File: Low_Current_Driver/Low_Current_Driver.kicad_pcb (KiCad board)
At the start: 4 copper layers, 160 x 99.5 mm, 194 parts, among them J1 Conn_01x02, J2 RJ45, J3 Screw_Terminal_01x04, J4 Conn_02x07_Odd_Even, J5 Channel 3, J6 Channel 2, J7 Channel 1, J8 MS548-10F, J9 Conn_01x02, Q1 Si4447ADY, Q2 IRF8707PbF, SW1 DPDT_Hirose, U1 LM4040DBZ-5, U10 OPA2210, U11 OPA2210, U12 OPA2210, U13 OPA2210, U14 OPA2210, U2 LM4040DBZ-5, U3 LM393, U4 TPS7A470x, U5 TPS7A470x, U6 TPS7A33, U7 LTC6655-2.5, U8 DAC8814, U9 OPA2210

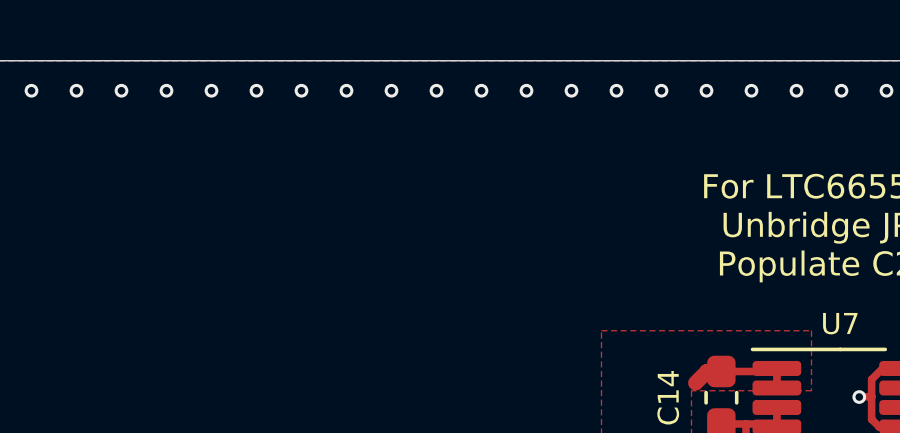
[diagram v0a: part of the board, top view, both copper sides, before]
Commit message: Revert "LCD amplifier update"
This reverts commit 83ce83a7733d65f451b9b157d86b817c7c87638f.
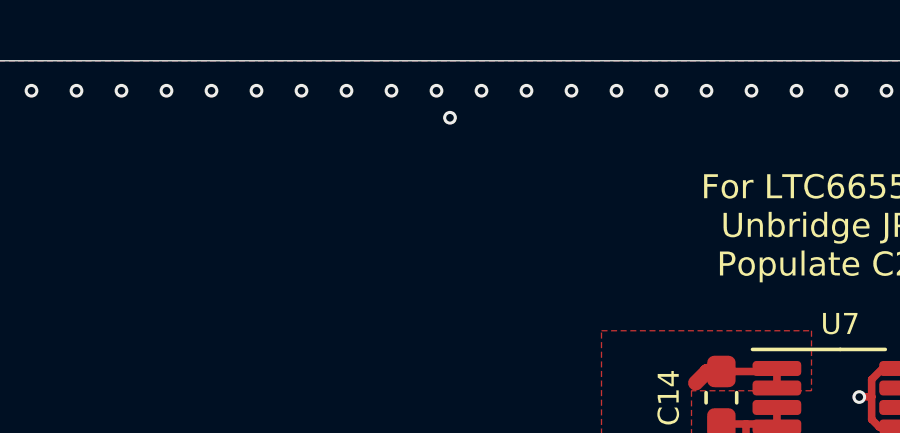
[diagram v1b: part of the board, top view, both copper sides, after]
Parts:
- U10, U11, U12, U13, U14, U9: value OPA2210 -> OPA2277
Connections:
- A1 pad 1: (no net) -> Net-(A1-Pad1)
- A1 pad 17: (no net) -> Net-(A1-Pad17)
- A1 pad 18: (no net) -> Net-(A1-Pad18)
- A1 pad 2: (no net) -> Net-(A1-Pad2)
- A1 pad 20: (no net) -> Net-(A1-Pad20)
- A1 pad 21: (no net) -> Net-(A1-Pad21)
- A1 pad 22: (no net) -> Net-(A1-Pad22)
- A1 pad 23: (no net) -> Net-(A1-Pad23)
- A1 pad 24: (no net) -> Net-(A1-Pad24)
- A1 pad 25: (no net) -> Net-(A1-Pad25)
- A1 pad 26: (no net) -> Net-(A1-Pad26)
- A1 pad 28: (no net) -> Net-(A1-Pad28)
- A1 pad 3: (no net) -> Net-(A1-Pad3)
- A1 pad 5: (no net) -> Net-(A1-Pad5)
- A1 pad 6: (no net) -> Net-(A1-Pad6)
- A1 pad 7: (no net) -> Net-(A1-Pad7)
- A1 pad 8: (no net) -> Net-(A1-Pad8)
- A1 pad 9: (no net) -> Net-(A1-Pad9)
- U4 pad 11: (no net) -> Net-(U4-Pad11)
- U4 pad 4: (no net) -> Net-(U4-Pad4)
- U4 pad 5: (no net) -> Net-(U4-Pad5)
- U5 pad 11: (no net) -> Net-(U5-Pad11)
- U5 pad 12: (no net) -> Net-(U5-Pad12)
- U5 pad 4: (no net) -> Net-(U5-Pad4)
- U5 pad 5: (no net) -> Net-(U5-Pad5)
- U5 pad 8: (no net) -> Net-(U5-Pad8)
- U5 pad 9: (no net) -> Net-(U5-Pad9)
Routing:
- net (no net): vias 0 -> 1

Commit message: LCD amplifier update
-Updated OPA2277 originally on the schematic to what was actually used on the board (OPA2210)
-Added a DNP on one of the power mux diodes
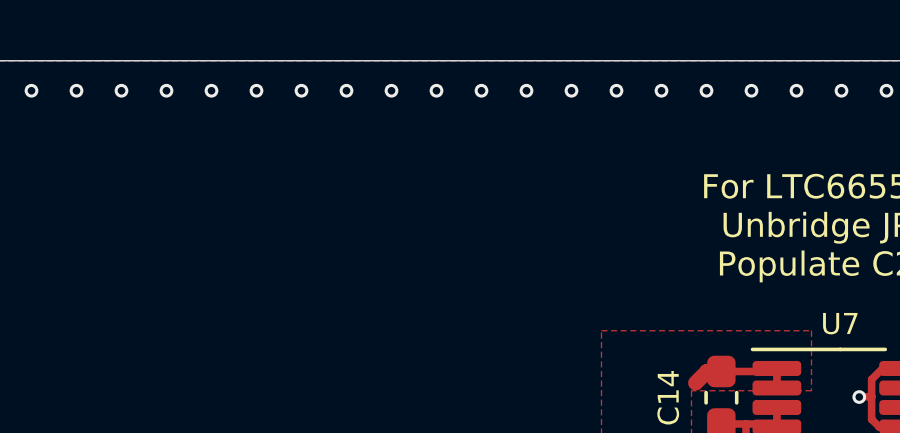
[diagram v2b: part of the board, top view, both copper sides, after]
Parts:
- U10, U11, U12, U13, U14, U9: value OPA2277 -> OPA2210
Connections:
- A1 pad 1: Net-(A1-Pad1) -> (no net)
- A1 pad 17: Net-(A1-Pad17) -> (no net)
- A1 pad 18: Net-(A1-Pad18) -> (no net)
- A1 pad 2: Net-(A1-Pad2) -> (no net)
- A1 pad 20: Net-(A1-Pad20) -> (no net)
- A1 pad 21: Net-(A1-Pad21) -> (no net)
- A1 pad 22: Net-(A1-Pad22) -> (no net)
- A1 pad 23: Net-(A1-Pad23) -> (no net)
- A1 pad 24: Net-(A1-Pad24) -> (no net)
- A1 pad 25: Net-(A1-Pad25) -> (no net)
- A1 pad 26: Net-(A1-Pad26) -> (no net)
- A1 pad 28: Net-(A1-Pad28) -> (no net)
- A1 pad 3: Net-(A1-Pad3) -> (no net)
- A1 pad 5: Net-(A1-Pad5) -> (no net)
- A1 pad 6: Net-(A1-Pad6) -> (no net)
- A1 pad 7: Net-(A1-Pad7) -> (no net)
- A1 pad 8: Net-(A1-Pad8) -> (no net)
- A1 pad 9: Net-(A1-Pad9) -> (no net)
- U4 pad 11: Net-(U4-Pad11) -> (no net)
- U4 pad 4: Net-(U4-Pad4) -> (no net)
- U4 pad 5: Net-(U4-Pad5) -> (no net)
- U5 pad 11: Net-(U5-Pad11) -> (no net)
- U5 pad 12: Net-(U5-Pad12) -> (no net)
- U5 pad 4: Net-(U5-Pad4) -> (no net)
- U5 pad 5: Net-(U5-Pad5) -> (no net)
- U5 pad 8: Net-(U5-Pad8) -> (no net)
- U5 pad 9: Net-(U5-Pad9) -> (no net)
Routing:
- net (no net): vias 1 -> 0
